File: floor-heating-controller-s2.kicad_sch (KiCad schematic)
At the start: 24 parts, among them J1 Supply, J10 VALVE1, J11 VALVE2, J12 VALVE3, J13 VALVE4, J14 VALVE5, J15 VALVE6, J16 VALVE7, J17 VALVE8, J18 EXT, J2 DS18B20_1, J3 DS18B20_2, J4 DS18B20_3, J5 DS18B20_4, J6 DS18B20_5, J7 DS18B20_6, J8 DS18B20_7, J9 DS18B20_8, U1 CJ431, U2 WeMos_S2_mini

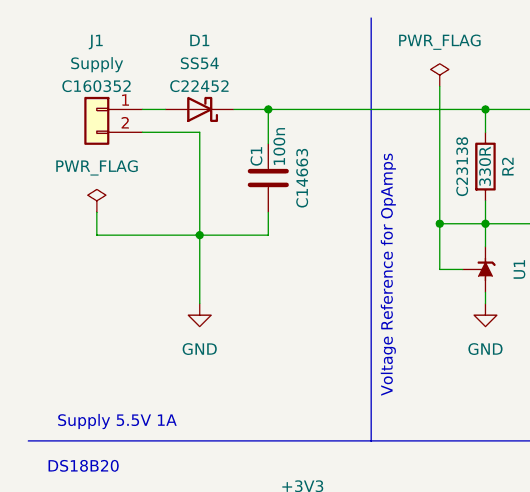
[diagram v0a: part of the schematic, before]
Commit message: production ready
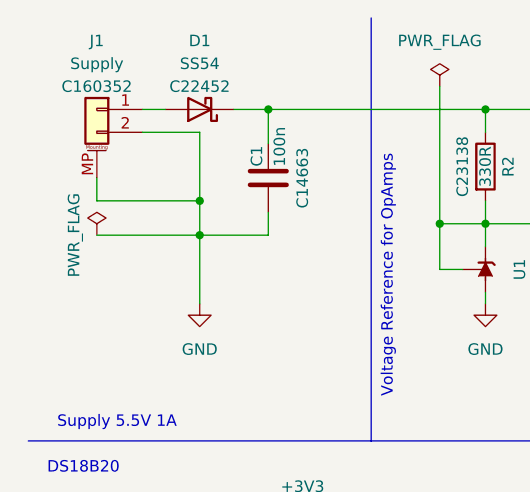
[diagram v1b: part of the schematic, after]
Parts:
- J1: symbol Connector_Generic:Conn_01x02 -> Connector_Generic_MountingPin:Conn_01x02_MountingPin
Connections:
- net GND: now also J1.MP (MountPin)
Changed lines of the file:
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@@
   (junction (at 133.35 143.51) (diameter 0) (color 0 0 0 0)
+  )
+  (junction (at 31.75 33.02) (diameter 0) (color 0 0 0 0)
   )
   (junction (at 91.44 173.99) (diameter 0) (color 0 0 0 0)
@@
     (stroke (width 0) (type default) (color 0 0 0 0))
   )
-  (wire (pts (xy 31.75 25.4) (xy 31.75 36.83))
+  (wire (pts (xy 20.32 33.02) (xy 31.75 33.02))
+    (stroke (width 0) (type default) (color 0 0 0 0))
+  )
+  (wire (pts (xy 31.75 25.4) (xy 31.75 33.02))
     (stroke (width 0) (type default) (color 0 0 0 0))
   )
@@
     (stroke (width 0) (type default) (color 0 0 0 0))
   )
+  (wire (pts (xy 93.98 69.85) (xy 105.41 69.85))
+    (stroke (width 0) (type default) (color 0 0 0 0))
+  )
   (wire (pts (xy 191.77 80.01) (xy 204.47 80.01))
     (stroke (width 0) (type default) (color 0 0 0 0))
@@
     (stroke (width 0) (type default) (color 0 0 0 0))
   )
+  (wire (pts (xy 31.75 33.02) (xy 31.75 36.83))
+    (stroke (width 0) (type default) (color 0 0 0 0))
+  )
   (wire (pts (xy 21.59 147.32) (xy 33.02 147.32))
     (stroke (width 0) (type default) (color 0 0 0 0))
@@
     (stroke (width 0) (type default) (color 0 0 0 0))
   )
+  (wire (pts (xy 20.32 30.48) (xy 20.32 33.02))
+    (stroke (width 0) (type default) (color 0 0 0 0))
+  )
   (polyline (pts (xy 176.53 12.7) (xy 176.53 166.37))
     (stroke (width 0) (type default) (color 0 0 0 0))
@@
     (stroke (width 0) (type default) (color 0 0 0 0))
   )
-  (wire (pts (xy 20.32 36.83) (xy 20.32 34.29))
-    (stroke (width 0) (type default) (color 0 0 0 0))
-  )
   (wire (pts (xy 242.57 128.27) (xy 242.57 125.73))
     (stroke (width 0) (type default) (color 0 0 0 0))
@@
   )
   (wire (pts (xy 71.12 35.56) (xy 71.12 20.32))
-    (stroke (width 0) (type default) (color 0 0 0 0))
-  )
-  (wire (pts (xy 93.98 69.85) (xy 105.41 69.85))
     (stroke (width 0) (type default) (color 0 0 0 0))
   )
@@
     )
   )
-  (symbol (lib_id "power:PWR_FLAG") (at 20.32 34.29 0) (unit 1)
-    (in_bom yes) (on_board yes) (fields_autoplaced)
-    (property "Reference" "#FLG0103" (id 0) (at 20.32 32.385 0)
-      (effects (font (size 1.27 1.27)) hide)
-    )
-    (property "Value" "PWR_FLAG" (id 1) (at 20.32 29.21 0))
-    (property "Footprint" "" (id 2) (at 20.32 34.29 0)
-      (effects (font (size 1.27 1.27)) hide)
-    )
-    (property "Datasheet" "~" (id 3) (at 20.32 34.29 0)
+  (symbol (lib_id "power:PWR_FLAG") (at 20.32 36.83 0) (unit 1)
+    (in_bom yes) (on_board yes)
+    (property "Reference" "#FLG0103" (id 0) (at 20.32 34.925 0)
+      (effects (font (size 1.27 1.27)) hide)
+    )
+    (property "Value" "PWR_FLAG" (id 1) (at 17.78 36.83 90))
+    (property "Footprint" "" (id 2) (at 20.32 36.83 0)
+      (effects (font (size 1.27 1.27)) hide)
+    )
+    (property "Datasheet" "~" (id 3) (at 20.32 36.83 0)
       (effects (font (size 1.27 1.27)) hide)
     )
@@
     (pin "MP")
   )
-  (symbol (lib_id "Connector_Generic:Conn_01x02") (at 20.32 22.86 0) (mirror y) (unit 1)
+  (symbol (lib_id "Connector_Generic_MountingPin:Conn_01x02_MountingPin") (at 20.32 22.86 0) (mirror y) (unit 1)
     (in_bom yes) (on_board yes)
     (property "Reference" "J1" (id 0) (at 20.32 15.24 0))
@@
     (pin "1")
     (pin "2")
+    (pin "MP")
   )
   (symbol (lib_id "power:+5V") (at 33.02 106.68 0) (unit 1)
